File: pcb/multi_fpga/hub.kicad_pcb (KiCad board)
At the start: 2 copper layers, 131.8 x 128.5 mm, 24 parts, among them J1 PinSocket_2x06_P2.54mm_Vertic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, J2 PinSocket_2x06_P2.54mm_Vertic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, J3 PinSocket_2x06_P2.54mm_Vertic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, J4 PinSocket_2x06_P2.54mm_Vertic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, J5 PinSocket_1x02_P2.54mm_Vertic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, J6 PinSocket_1x02_P2.54mm_Vertic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, J7 PinSocket_1x02_P2.54mm_Vertic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, J8 PinSocket_1x02_P2.54mm_Vertic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, Y1 TCXO_Can

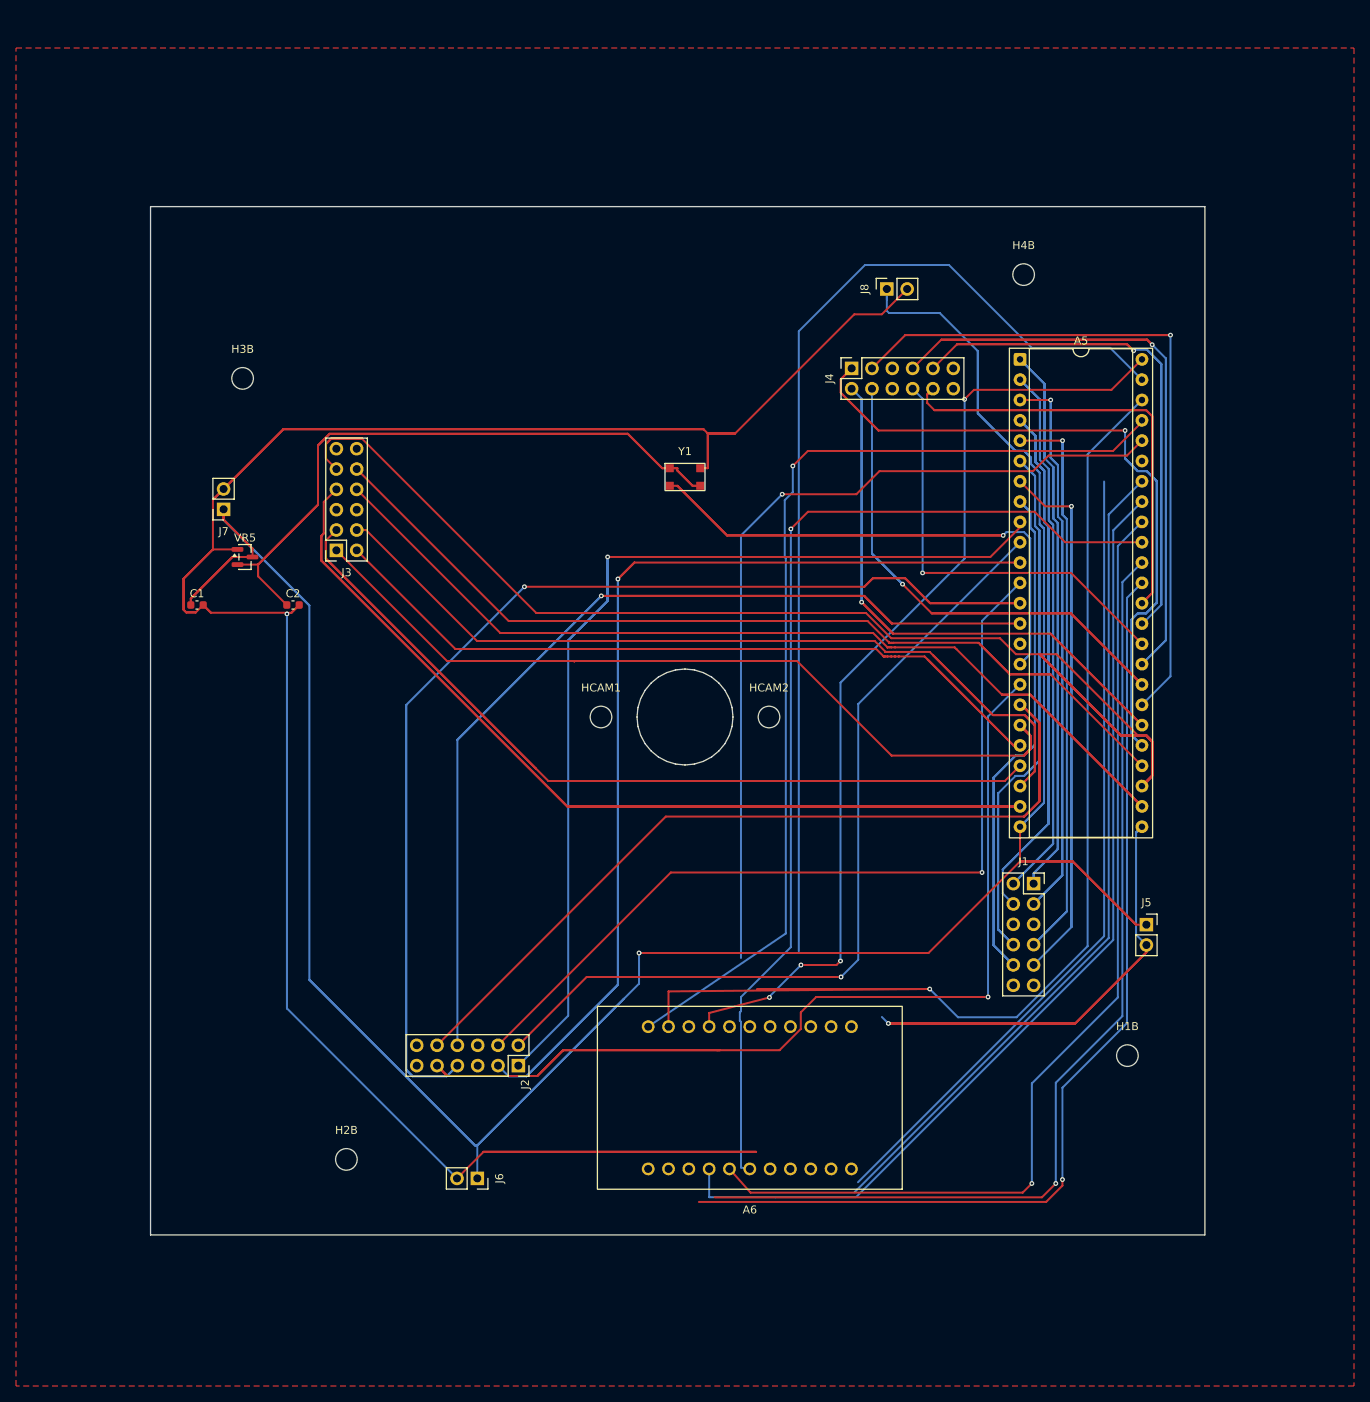
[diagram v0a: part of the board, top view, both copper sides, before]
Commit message: Manually routed. DRC-clean.
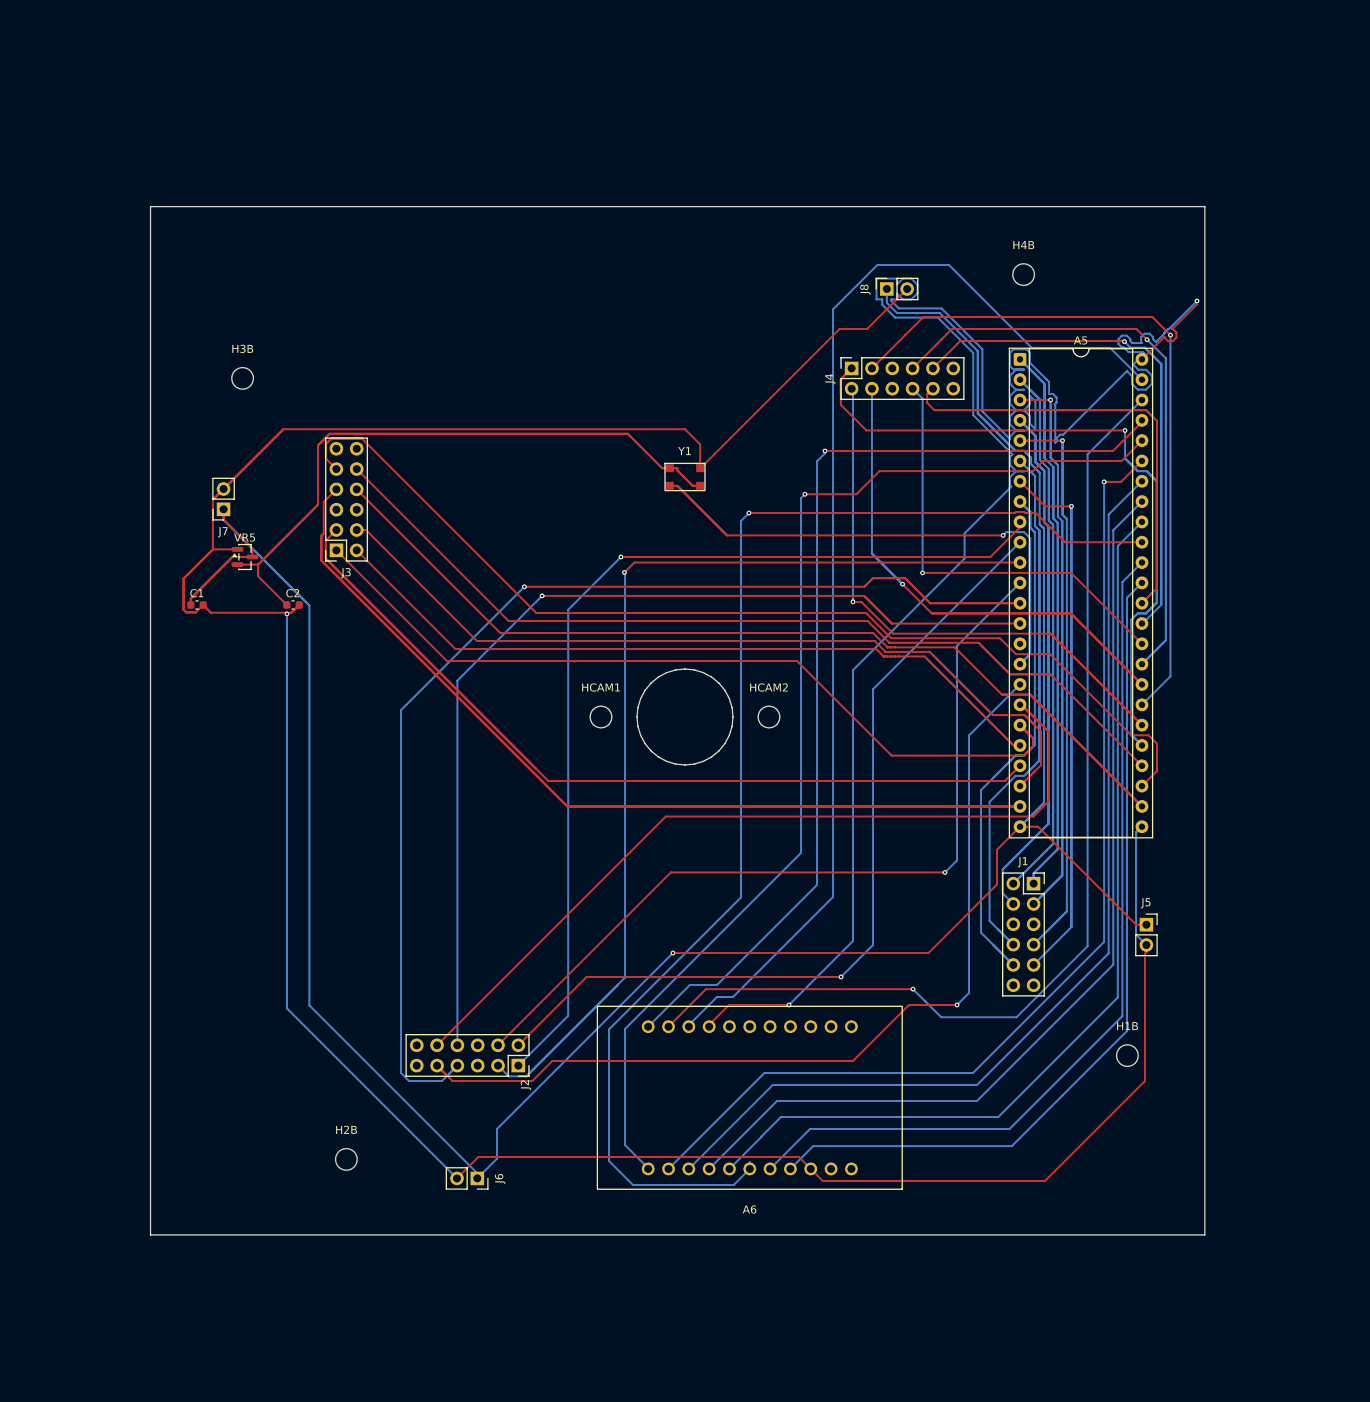
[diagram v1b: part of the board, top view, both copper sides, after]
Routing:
- net SPOKE2_STROBE: track 299.3 -> 141.1 mm
- net USB_WR_N: track 121.2 -> 266.9 mm, vias 4 -> 2
- net GND: track 553.2 -> 433.7 mm, vias 2 -> 1
- net +5V: track 468.1 -> 397.6 mm
- net SPOKE1_D5: track 180.6 -> 126.6 mm
- net SPOKE1_D2: track 191.9 -> 138.4 mm
- net SPOKE1_D4: track 211.6 -> 162.2 mm
- net TCXO_CLK: track 109.5 -> 75.0 mm
- net USB_D7: track 107.8 -> 139.8 mm
- net SPOKE3_D2: track 119.9 -> 88.6 mm
- net SPOKE3_D1: track 115.8 -> 85.4 mm
- net USB_D2: track 130.0 -> 159.6 mm
- net USB_D6: track 100.3 -> 129.6 mm, vias 0 -> 1
- net SPOKE1_STROBE: track 141.8 -> 114.9 mm
- net SPOKE3_D4: track 139.6 -> 114.1 mm
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- removed copper zone on F.Cu, net GND
